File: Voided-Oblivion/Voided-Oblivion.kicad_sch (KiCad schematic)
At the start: 86 parts, among them J1 Top male, J10 Sub-Module TL, J11 Sub-Module LT, J12 Sub-Module TR, J16 Sub-Module BL, J17 Sub-Module LB, J18 Sub-Module BR, J19 Sub-Module RB, J2 Top female, J20 Sub-Module RT, J3 Right male, J4 Right female, J5 Left male, J6 Left female, J7 Bottom male, J8 Bottom female, J9 SM03B-SRSS-TB, SW1 boot, SW2 reset, U1 RP2350_80QFN, U3 W25Q128JVS, U4 W25Q128JVS, Y1 ABM8-272-T3

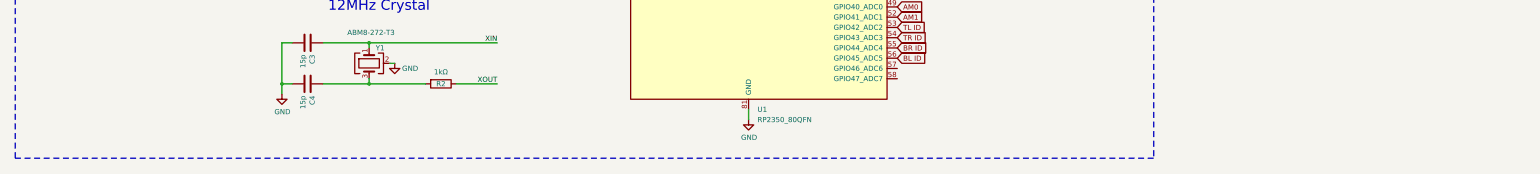
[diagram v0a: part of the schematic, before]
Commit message: checkpoint
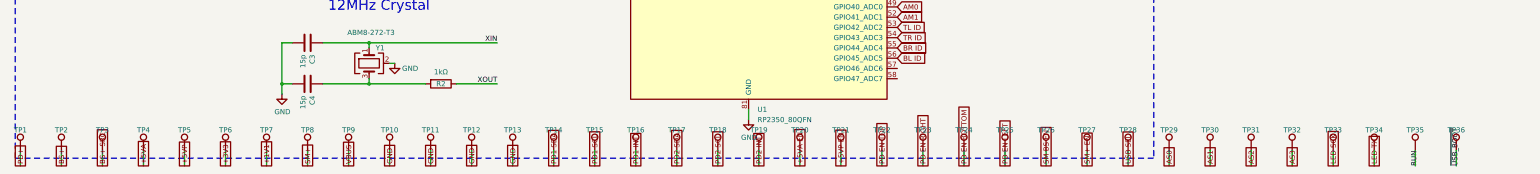
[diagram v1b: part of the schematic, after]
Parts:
- added TP1, TP10, TP11, TP12, TP13, TP14, TP15, TP16, TP17, TP18, TP19, TP2, TP20, TP21, TP22, TP23, TP24, TP25, TP26, TP27, TP28, TP29, TP3, TP30, TP31, TP32, TP33, TP34, TP35, TP36, TP4, TP5, TP6, TP7, TP8, TP9: TestPoint, TestPoint:TestPoint_Pad_D1.0mm, symbol Connector:TestPoint
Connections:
- net +1V1: now also TP7.1
- net +3V3: now also TP6.1
- net +5VP EN: now also TP21.1
- net AS0: now also TP29.1
- net AS1: now also TP30.1
- net AS2: now also TP31.1
- net AS3: now also TP32.1
- net BS+: now also TP2.1
- net BS+ SRC: now also TP3.1
- net GND: now also TP10.1, TP11.1, TP12.1, TP13.1
- net LED SCK: now also TP33.1
- net LED TX: now also TP34.1
- net PD EN BOTTOM: now also TP24.1
- net PD EN LEFT: now also TP25.1
- net PD EN RIGHT: now also TP23.1
- net PD EN TOP: now also TP22.1
- net PD1 INT: now also TP16.1
- net PD1 SCL: now also TP15.1
- net PD1 SDA: now also TP14.1
- net PD2 INT: now also TP19.1
- net PD2 SCL: now also TP18.1
- net PD2 SDA: now also TP17.1
- net RUN: now also TP35.1
- net SM BS EN: now also TP26.1
- net SM+: now also TP8.1
- net SM+ EN: now also TP27.1
- net ~{USB_BOOT}: now also TP36.1
- new net +5VA: TP4.1
- new net +5VA EN: TP20.1
- new net +5VP: TP5.1
- new net PD+: TP1.1
- new net USB SEL: TP28.1
- new net VBUS: TP9.1
